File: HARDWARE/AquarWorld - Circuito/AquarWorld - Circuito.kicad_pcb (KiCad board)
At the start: 2 copper layers, 158.6 x 90.8 mm, 80 parts, among them J10 SALIDA - RELAY 1, J13 12V - GND, J15 5V - GND, J2 MP3-PLAYER, J27 ALIMENTACIÓN - 12V, J3 SENSOR DE TEMPERATURA, J4 SALIDA - RELAY 2, J5 SENSOR ULTRASONICO, J6 SALIDA - RELAY 3, J7 SALIDA - RELAY 4, K1 RELAY 2, K2 RELAY 3, K3 RELAY 4, K5 RELAY 1, Q1 2N7000, Q2 2N7000, Q3 2N7000, Q4 2N7000, Q5 2N7000, SW1 PULSADOR 1, SW4 PULSADOR 2, SW7 PULSADOR 3, U1 PC817, U2 DEVKIT_V1_ESP32-WROOM-32, U3 PC817, U5 PC817, U6 L7805, U7 PC817

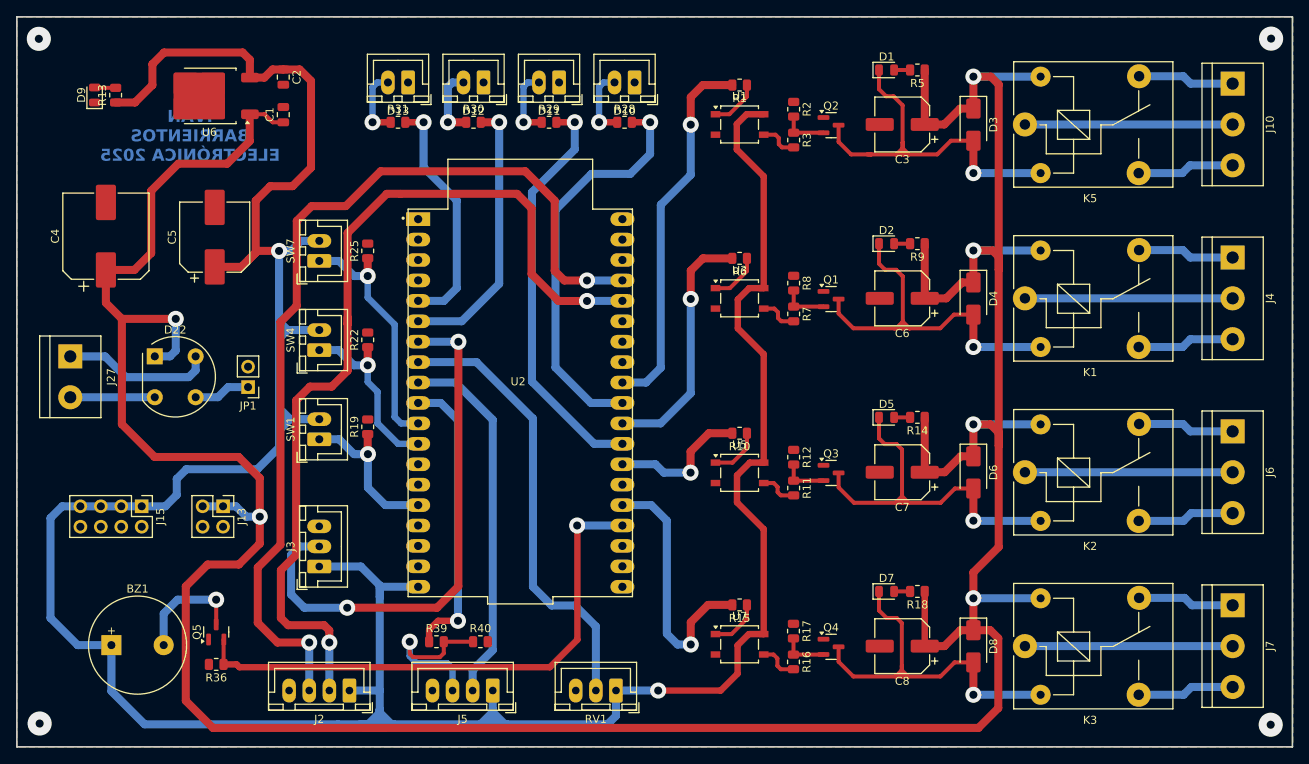
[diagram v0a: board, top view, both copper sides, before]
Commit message: Placa pricipal - AquarWorld
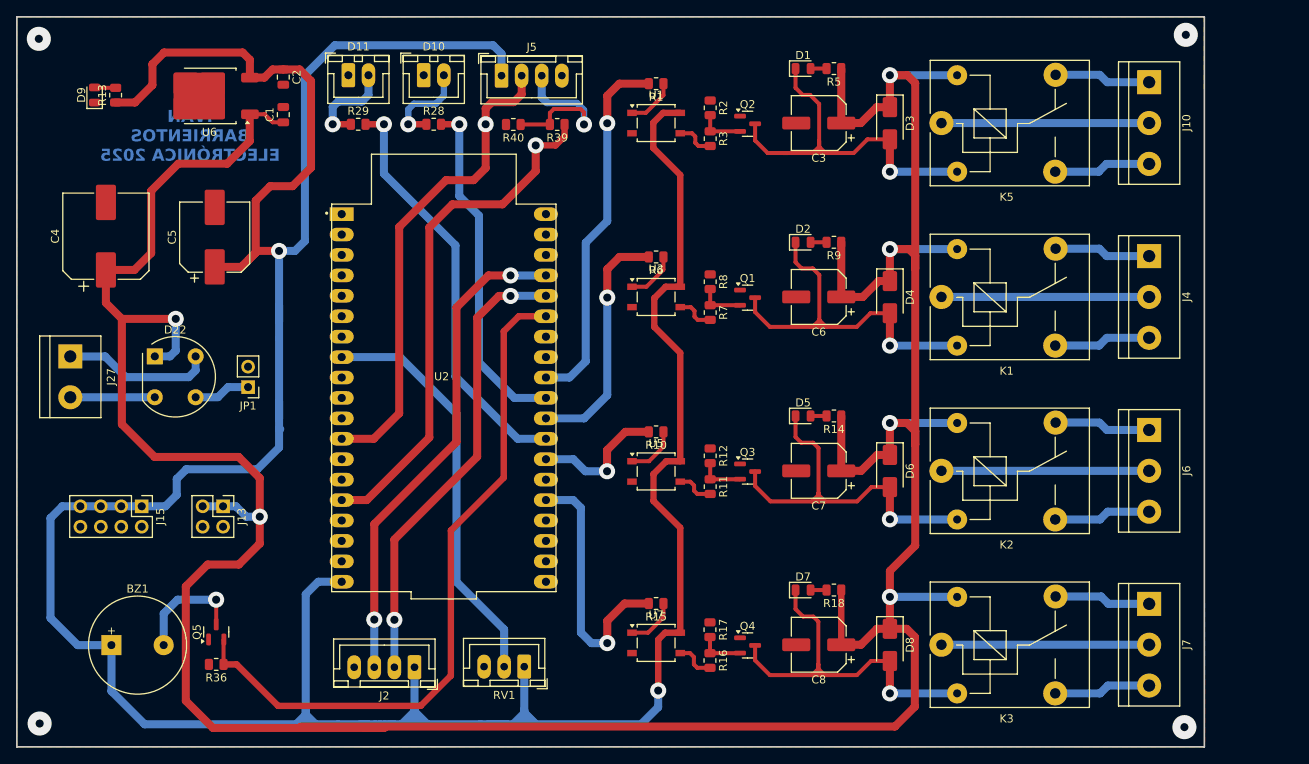
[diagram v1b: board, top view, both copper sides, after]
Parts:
- removed D12, D13: LED, Connector_JST:JST_XH_B2B-XH-A_1x02_P2.50mm_Vertical
- removed J3: SENSOR DE TEMPERATURA, Connector_JST:JST_XH_B3B-XH-A_1x03_P2.50mm_Vertical
- removed R19, R22, R25: 1KΩ, Resistor_SMD:R_0805_2012Metric
- removed R30, R31: 220Ω, Resistor_SMD:R_0805_2012Metric
- removed SW1: PULSADOR 1, Connector_JST:JST_XH_B2B-XH-A_1x02_P2.50mm_Vertical
- removed SW4: PULSADOR 2, Connector_JST:JST_XH_B2B-XH-A_1x02_P2.50mm_Vertical
- removed SW7: PULSADOR 3, Connector_JST:JST_XH_B2B-XH-A_1x02_P2.50mm_Vertical
- moved J5 76.5 mm to (126.6, 53.1), turned to 0 degrees
- moved R39 66.1 mm to (133.6, 59.1), turned to 180 degrees
- moved R40 64.5 mm to (128.1, 59.1), turned to 180 degrees
- moved D10 26.2 mm to (117.0, 53.0), turned to 0 degrees
- moved D11 26.2 mm to (107.6, 53.0), turned to 0 degrees
- moved R28 23.7 mm to (118.2, 59.1)
- moved R29 23.7 mm to (108.8, 59.1)
- moved RV1 11.8 mm to (129.4, 126.6)
- moved C3 10.4 mm to (166.1, 59.0)
- moved C6 10.4 mm to (166.1, 80.6)
- moved C7 10.4 mm to (166.1, 102.2)
- moved C8 10.4 mm to (166.1, 123.9)
- moved R11 10.4 mm to (152.6, 104.2)
- moved R12 10.4 mm to (152.6, 100.4)
- moved R2 10.4 mm to (152.6, 57.1)
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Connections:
- U2 pad 10: ECHO -> unconnected-(U2-IO26-Pad10)
- U2 pad 11: PULSADOR 3 -> unconnected-(U2-IO27-Pad11)
- U2 pad 12: PULSADOR 2 -> TRIG
- U2 pad 15: PULSADOR 1 -> ECHO
- U2 pad 23: BUZZER -> unconnected-(U2-IO15-Pad23)
- U2 pad 33: unconnected-(U2-IO21-Pad33) -> BUZZER
- U2 pad 5: LED - ADVERTENCIA 4 -> unconnected-(U2-IO34-Pad5)
- U2 pad 6: LED - ADVERTENCIA 3 -> unconnected-(U2-IO35-Pad6)
- U2 pad 7: SENSOR DE TEMPERATURA -> unconnected-(U2-IO32-Pad7)
- U2 pad 9: TRIG -> unconnected-(U2-IO25-Pad9)
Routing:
- net SENSOR DE TEMPERATURA: track 66.9 -> 0.00 mm, vias 2 -> 0
- net RX0: track 119.2 -> 61.8 mm
- net TX0: track 114.3 -> 57.4 mm
- net LED - ADVERTENCIA 3: track 34.4 -> 0.00 mm, vias 1 -> 0
- net PULSADOR 3: track 31.2 -> 0.00 mm, vias 1 -> 0
- net LED - ADVERTENCIA 4: track 30.1 -> 0.00 mm, vias 1 -> 0
- net ECHO: track 36.3 -> 65.1 mm
- net PULSADOR 2: track 23.1 -> 0.00 mm, vias 1 -> 0
- net +5V: track 400.6 -> 421.3 mm
- net PULSADOR 1: track 20.6 -> 0.00 mm, vias 1 -> 0
- net BUZZER: track 69.4 -> 86.6 mm, vias 1 -> 0
- net TRIG: track 45.9 -> 60.4 mm, vias 0 -> 1
- net Net-(D12-A): track 8.83 -> 0.00 mm, vias 1 -> 0
- net Net-(D13-A): track 8.78 -> 0.00 mm, vias 1 -> 0
- net LED - ADVERTENCIA 1: track 50.6 -> 43.1 mm
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- removed copper zone on B.Cu, net Earth
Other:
- board size 158.6 x 90.8 mm -> 147.7 x 90.8 mm
